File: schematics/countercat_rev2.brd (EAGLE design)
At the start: 101.6 x 76.2 mm, 57 parts, among them IC1 74LS595N, Q2 2N3904, Q3 IRF520, Q4 IRF520, U4 ATMEGA328P_PDIP, U6 RELAYPTH3, Y1 16MHz

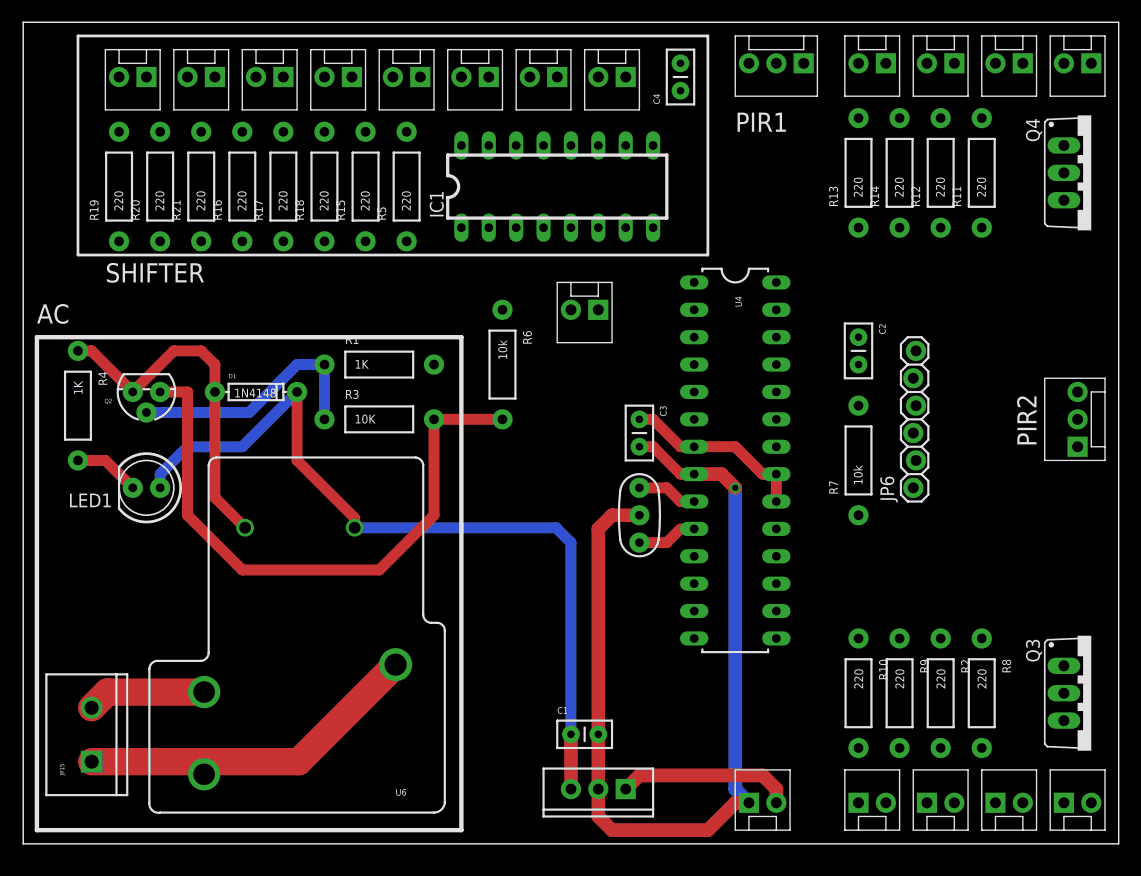
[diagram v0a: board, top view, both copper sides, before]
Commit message: Updated board and schematic
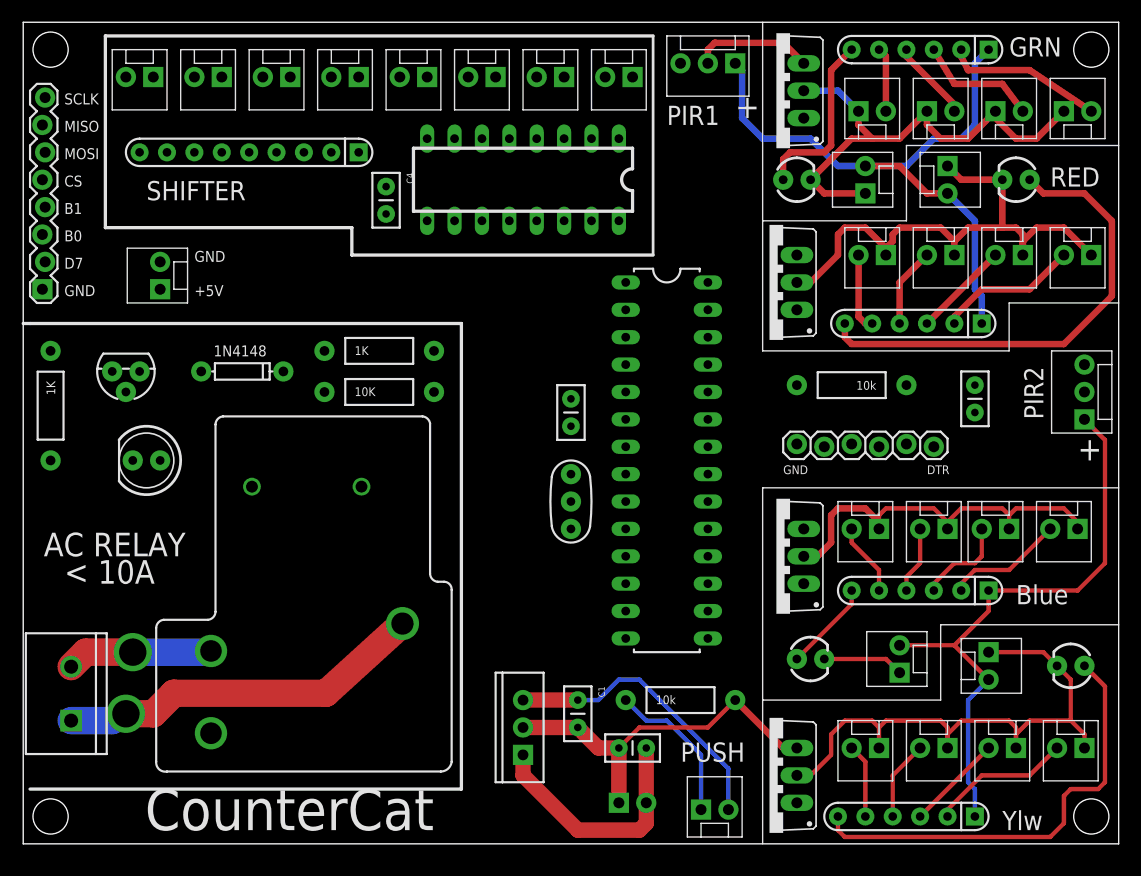
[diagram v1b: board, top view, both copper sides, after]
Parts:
- removed R10, R12, R13, R14, R15, R16, R17, R18, R19, R20, R21, R5: 220, SparkFun-Resistors:AXIAL-0.4
- added BLU, GRN, RED, YLW: (no value), SparkFun-LED:LED3MM
- added C5: .1uF, SparkFun-Capacitors:CAP-PTH-SMALL2
- added JP10: RED_RAW, SparkFun:MOLEX-1X2
- added JP24: GRN_RAW, SparkFun:MOLEX-1X2
- added JP25: BLU1, SparkFun:MOLEX-1X2
- added JP26: BLU2, SparkFun:MOLEX-1X2
- added JP27: BLU3, SparkFun:MOLEX-1X2
- added JP28: BLU4, SparkFun:MOLEX-1X2
- added JP29: BLU_RAW, SparkFun:MOLEX-1X2
- added JP30: YLW1, SparkFun:MOLEX-1X2
- added JP31: YLW2, SparkFun:MOLEX-1X2
- added JP32: YLW3, SparkFun:MOLEX-1X2
- added JP33: YLW4, SparkFun:MOLEX-1X2
- added JP34: YLW_RAW, SparkFun:MOLEX-1X2
- added JP35: AUX, SparkFun-Connectors:1X08_LOCK
- added JP36: AUX_PWR, SparkFun:MOLEX-1X2
- added Q1, Q5: IRF520, transistor-power:TO220BV
- added R35: R-GRN, SparkFun-Resistors:RPACK-SIP-PTH-5
- JP16: value RED1 -> SHF3
- JP17: value RED1 -> SHF5
- JP18: value RED1 -> SHF1
- JP19: value RED1 -> SHF2
- JP2: value RED1 -> SHF4
- JP20: value RED1 -> SHF8
- JP21: value RED1 -> SHF7
- JP22: value RED1 -> SHF6
- R11: value 220 -> R-SHF; device SparkFun-Resistors:AXIAL-0.4 -> SparkFun-Resistors:RPACK-SIP-PTH-8
- R2: value 220 -> R-RED; device SparkFun-Resistors:AXIAL-0.4 -> SparkFun-Resistors:RPACK-SIP-PTH-5
- R8: value 220 -> R-BLU; device SparkFun-Resistors:AXIAL-0.4 -> SparkFun-Resistors:RPACK-SIP-PTH-5
- R9: value 220 -> R-YLW; device SparkFun-Resistors:AXIAL-0.4 -> SparkFun-Resistors:RPACK-SIP-PTH-5
- moved R11 57.8 mm to (31.1, 64.1), turned to 270 degrees
- moved JP3 51.6 mm to (99.1, 54.6), turned to 180 degrees
- moved JP4 50.9 mm to (92.7, 54.6), turned to 180 degrees
- moved JP7 50.9 mm to (86.4, 54.6), turned to 180 degrees
- moved JP8 50.9 mm to (80.0, 54.6), turned to 180 degrees
- moved JP9 47.3 mm to (62.9, 3.17), turned to 0 degrees
- moved R6 35.2 mm to (61.0, 13.3), turned to 0 degrees
- moved R2 34.5 mm to (88.9, 48.3)
- moved Q3 31.9 mm to (69.8, 26.7), turned to 90 degrees
- moved Q4 30.2 mm to (69.8, 69.8), turned to 90 degrees
- moved C4 28.7 mm to (33.7, 61.0), turned to 270 degrees
- moved JP18 19.7 mm to (56.5, 71.1)
- moved JP19 19.7 mm to (50.2, 71.1)
- moved JP2 18.4 mm to (37.5, 71.1)
- moved R9 13.4 mm to (88.3, 2.54)
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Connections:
- removed net N$22 (its old number): JP8.2, R10.P$2
- removed net SFW_RXI: U4.4
- removed net SFW_TXO: U4.5
- new net B0: JP35.3, U4.14
- new net B1: JP35.4, U4.15
- new net BLU: Q3.G, U4.4
- new net D7: JP35.2, U4.13
- new net N$12: JP4.2, R2.P$3
- new net N$18: JP7.2, R2.P$4
- new net N$34: BLU.K, JP25.1, JP26.1, JP27.1, JP28.1, JP29.1, Q3.D
- new net N$35: JP26.2, R8.P$3
- new net N$36: JP27.2, R8.P$4
- new net N$37: JP28.2, R8.P$5
- new net N$38: BLU.A, R8.P$6
- new net N$39: JP25.2, R8.P$2
- new net N$40: JP30.1, JP31.1, JP32.1, JP33.1, JP34.1, Q5.D, YLW.K
- new net N$41: JP31.2, R9.P$3
- new net N$42: JP32.2, R9.P$4
- new net N$43: JP33.2, R9.P$5
- new net N$44: R9.P$6, YLW.A
- new net N$45: GRN.A, R35.P$6
- new net N$46: JP30.2, R9.P$2
- new net SPI_MISO: JP35.7, U4.18
- new net SPI_MOSI: JP35.6, U4.17
- new net SPI_SCK: JP35.8, U4.19
- new net YLW: Q5.G, U4.5
- net 5V: now also JP10.2, JP24.2, JP29.2, JP34.2, JP36.1, R35.P$1; no longer JP6.4, R10.P$1, R11.P$1, R12.P$1, R13.P$1, R14.P$1
- net GND: now also C5.2, JP35.1, JP36.2, Q1.S, Q5.S, R11.P$1; no longer JP16.2, JP17.2, JP18.2, JP19.2, JP2.2, JP20.2, JP21.2, JP22.2
- net N$1: now also IC1.4, JP17.1; no longer IC1.9
- net N$10: now also JP18.2, R11.P$2; no longer JP2.1, R5.P$2
- net N$11: now also JP19.2, R11.P$3; no longer JP16.1, R15.P$2
- net N$13: now also R35.P$3; no longer R12.P$2
- net N$14: now also JP16.2, R11.P$4; no longer JP19.1, R16.P$2
- net N$15: now also R35.P$4; no longer R13.P$2
- net N$16: now also R35.P$5; no longer R14.P$2
- net N$17: now also JP2.2, R11.P$5; no longer JP18.1, R17.P$2
- net N$19: now also JP8.2, R2.P$5; no longer JP4.2, R8.P$2
- net N$2: now also JP10.1, Q1.D, RED.K; no longer Q3.D
- net N$20: now also JP17.2, R11.P$6; no longer JP17.1, R18.P$2
- net N$21: now also R2.P$6, RED.A; no longer JP7.2, R9.P$2
- net N$23: now also JP22.2, R11.P$7; no longer JP22.1, R19.P$2
- net N$24: now also JP21.2, R11.P$8; no longer JP21.1, R20.P$2
- net N$25: now also JP20.2, R11.P$9; no longer JP20.1, R21.P$2
- net N$26: now also JP18.1; no longer R5.P$1
- net N$27: now also JP19.1; no longer R15.P$1
- net N$28: now also JP16.1; no longer R16.P$1
- net N$29: now also JP2.1; no longer R17.P$1
- net N$30: now also IC1.6, JP21.1; no longer IC1.4, R18.P$1
- net N$31: now also JP22.1; no longer R19.P$1
- net N$32: now also IC1.7, JP20.1; no longer IC1.6, R20.P$1
- net N$33: now also JP6.4; no longer IC1.7, R21.P$1
- net N$4: now also GRN.K, JP24.1, Q4.D
- net N$5: now also R35.P$2; no longer R11.P$2
- net RED: now also Q1.G; no longer Q3.G
- net SPI_CS: now also JP35.5
- net VB: now also C5.1
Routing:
- net GND: track 143.0 -> 46.2 mm, vias 1 -> 0
- net 5V: track 75.4 -> 142.7 mm
- net N$40: track 0.00 -> 54.5 mm
- net N$2: track 0.00 -> 50.5 mm
- net N$4: track 0.00 -> 46.0 mm
- net N$21: track 0.00 -> 44.3 mm
- net N$34: track 0.00 -> 42.9 mm
- net N$44: track 0.00 -> 41.5 mm
- net COIL: track 32.7 -> 0.00 mm
- net N$6: track 23.4 -> 0.00 mm
- net N$8: track 17.3 -> 0.00 mm
- net N$45: track 0.00 -> 16.6 mm
- net N$5: track 0.00 -> 14.6 mm
- net PUSH: track 0.00 -> 14.2 mm
- net N$46: track 0.00 -> 13.2 mm
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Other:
- board text added: "+"
- board text added: "+5V"
- board text added: "< 10A"
- board text added: "AC RELAY"
- board text added: "B0"
- board text added: "B1"
- board text added: "Blue"
- board text added: "CS"
- board text added: "CounterCat"
- board text added: "D7"
- board text added: "DTR"
- board text added: "GND"
- board text added: "GRN"
- board text added: "MISO"
- board text added: "MOSI"
- board text added: "PUSH"
- board text added: "RED"
- board text added: "SCLK"
- board text added: "Ylw"
- board text removed: "AC"
